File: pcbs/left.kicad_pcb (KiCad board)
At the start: 2 copper layers, 123.1 x 93.2 mm, 29 parts

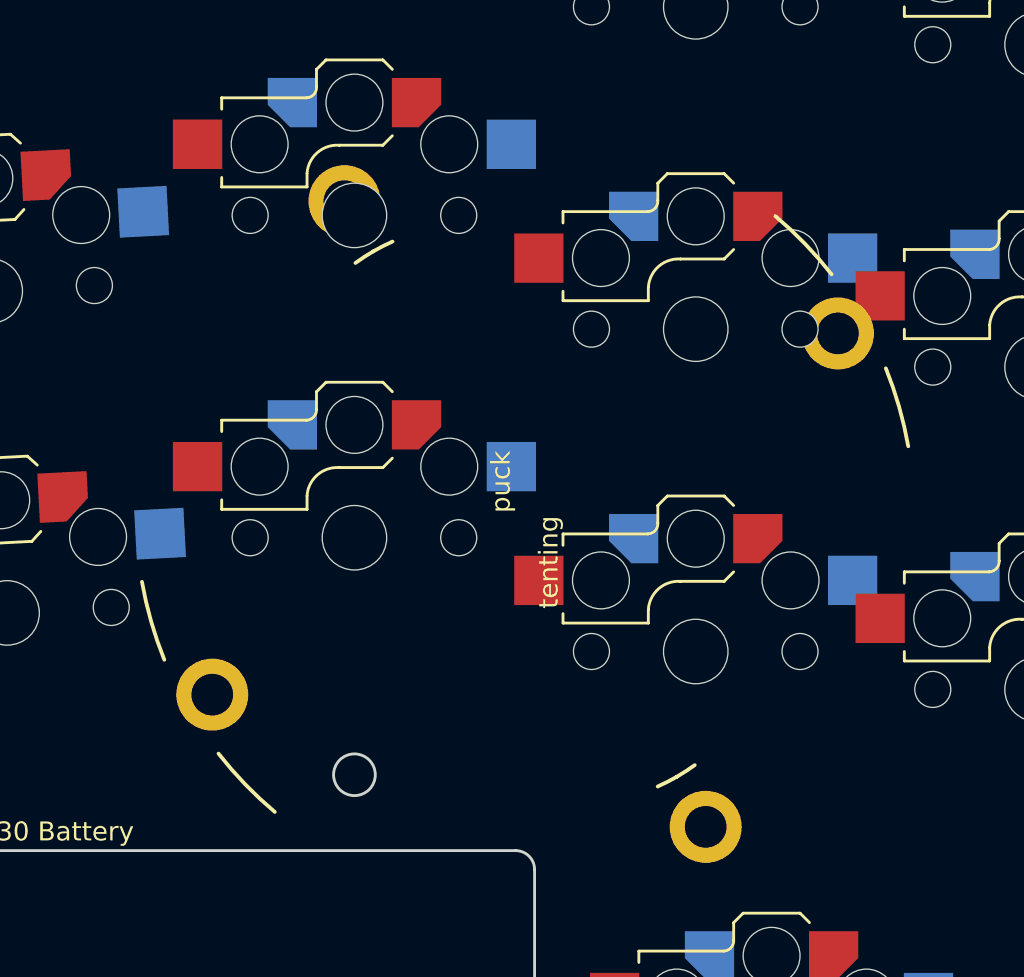
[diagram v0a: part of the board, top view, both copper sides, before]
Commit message: Tweak
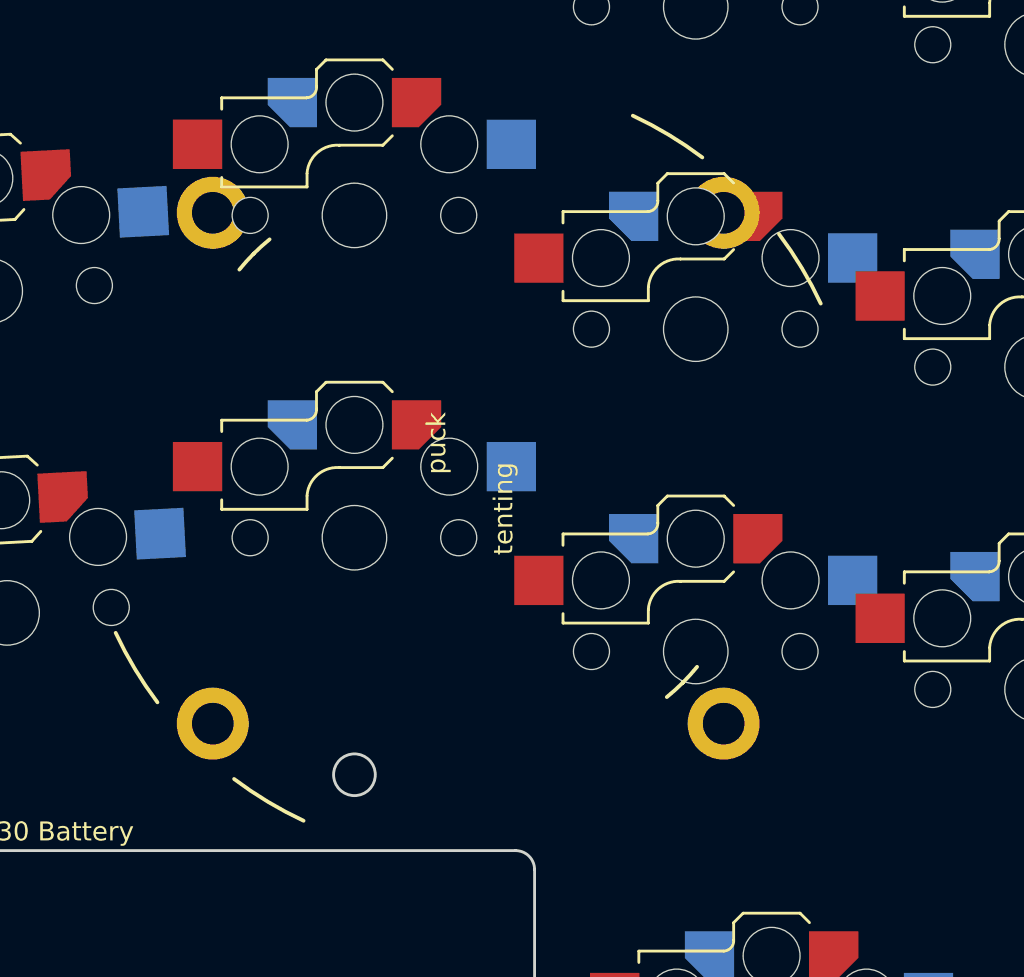
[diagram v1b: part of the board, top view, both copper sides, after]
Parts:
- moved TENTINGPUCK1 3.85 mm to (141.1, 75.5), turned to 45 degrees
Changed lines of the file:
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@@
 	(generator_version "8.0")
 	(layer "F.Cu")
-  (at 144.14836665 77.93429119999999 30)
+  (at 141.14836666666667 75.51762453333332 45)
 	(property "Reference" "TENTINGPUCK1"
 		(at 0 0 0)

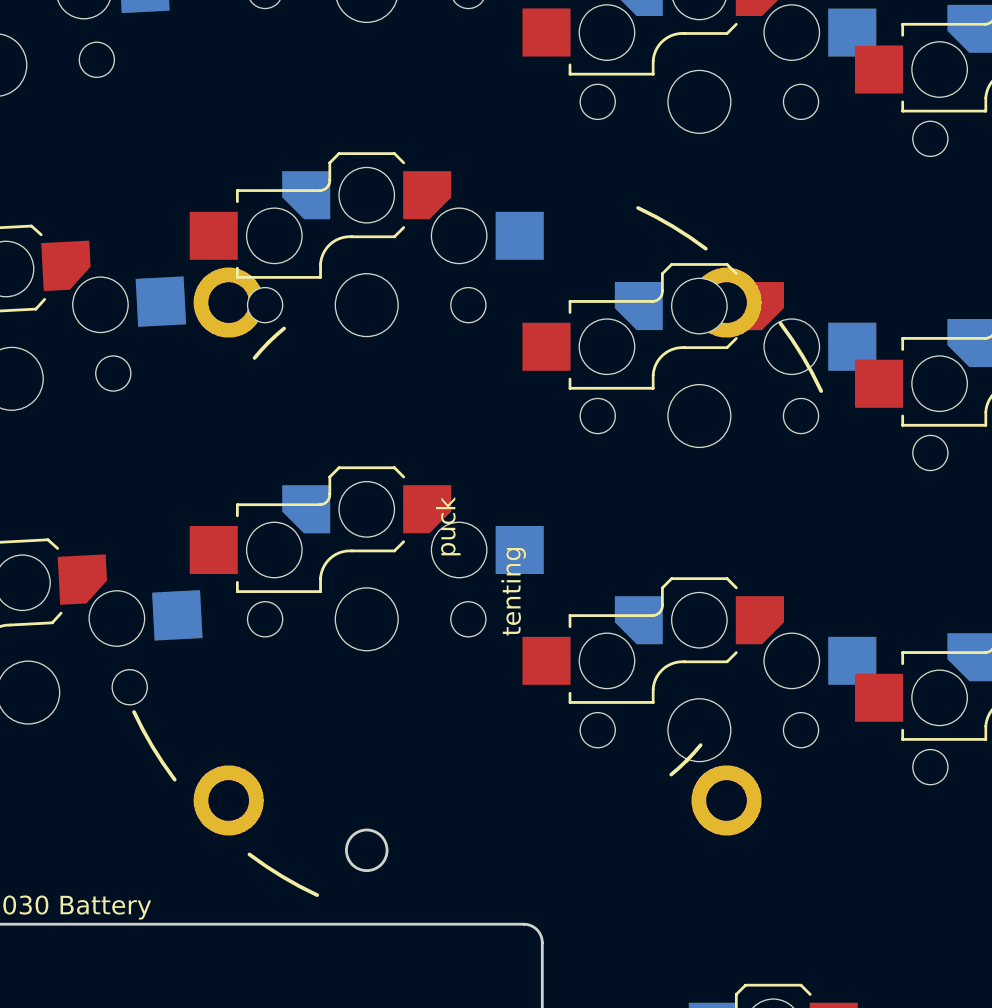
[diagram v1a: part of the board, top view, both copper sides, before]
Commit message: Dial it in
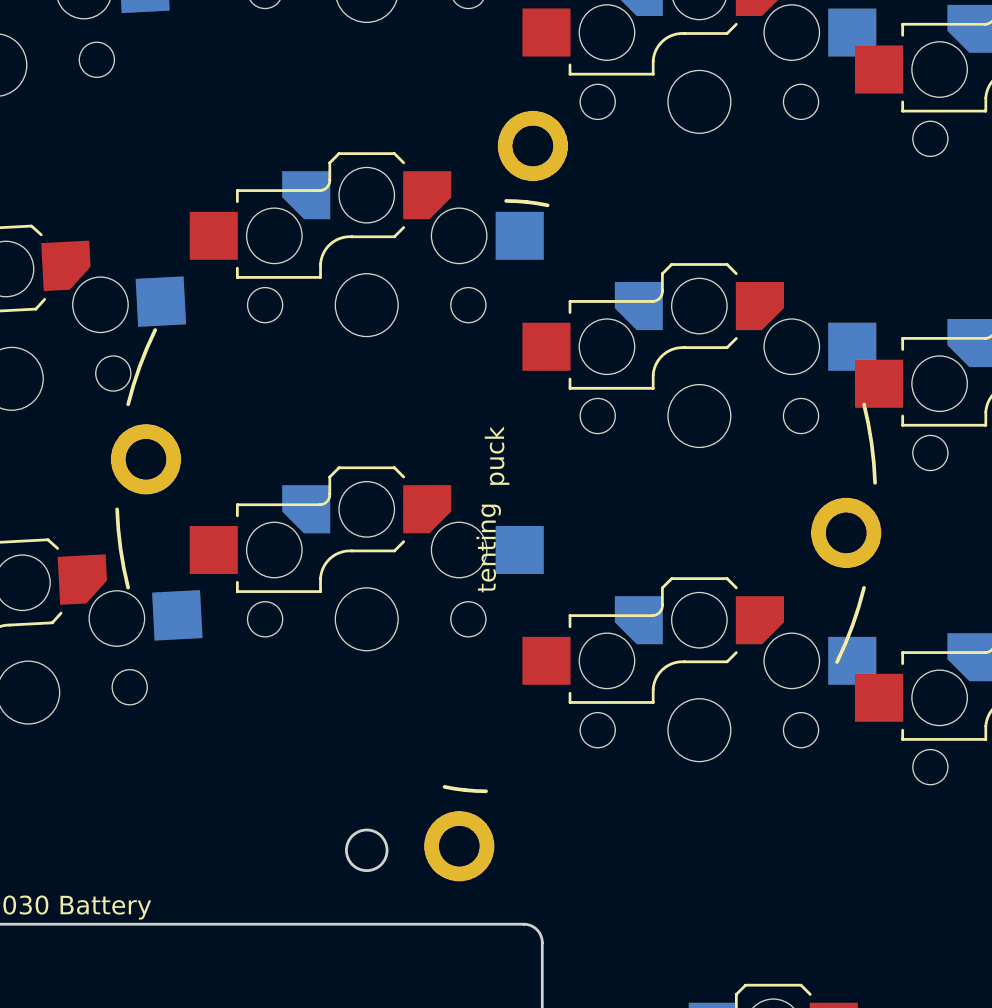
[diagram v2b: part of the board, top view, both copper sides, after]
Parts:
- moved TENTINGPUCK1 3.16 mm to (142.1, 72.5), turned to -6 degrees
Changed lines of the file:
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@@
 	(generator_version "8.0")
 	(layer "F.Cu")
-  (at 141.14836666666667 75.51762453333332 45)
+  (at 142.14836666666667 72.51762453333332 -6)
 	(property "Reference" "TENTINGPUCK1"
 		(at 0 0 0)
